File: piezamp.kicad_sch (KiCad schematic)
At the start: 54 parts, among them J3 Output (TRS), J4 Power_Conn, J5 Piezo A, J6 Piezo B, SW1 Power, SW2 Mode / Polarity, U1 NE5532DR, U2 NE5532DR

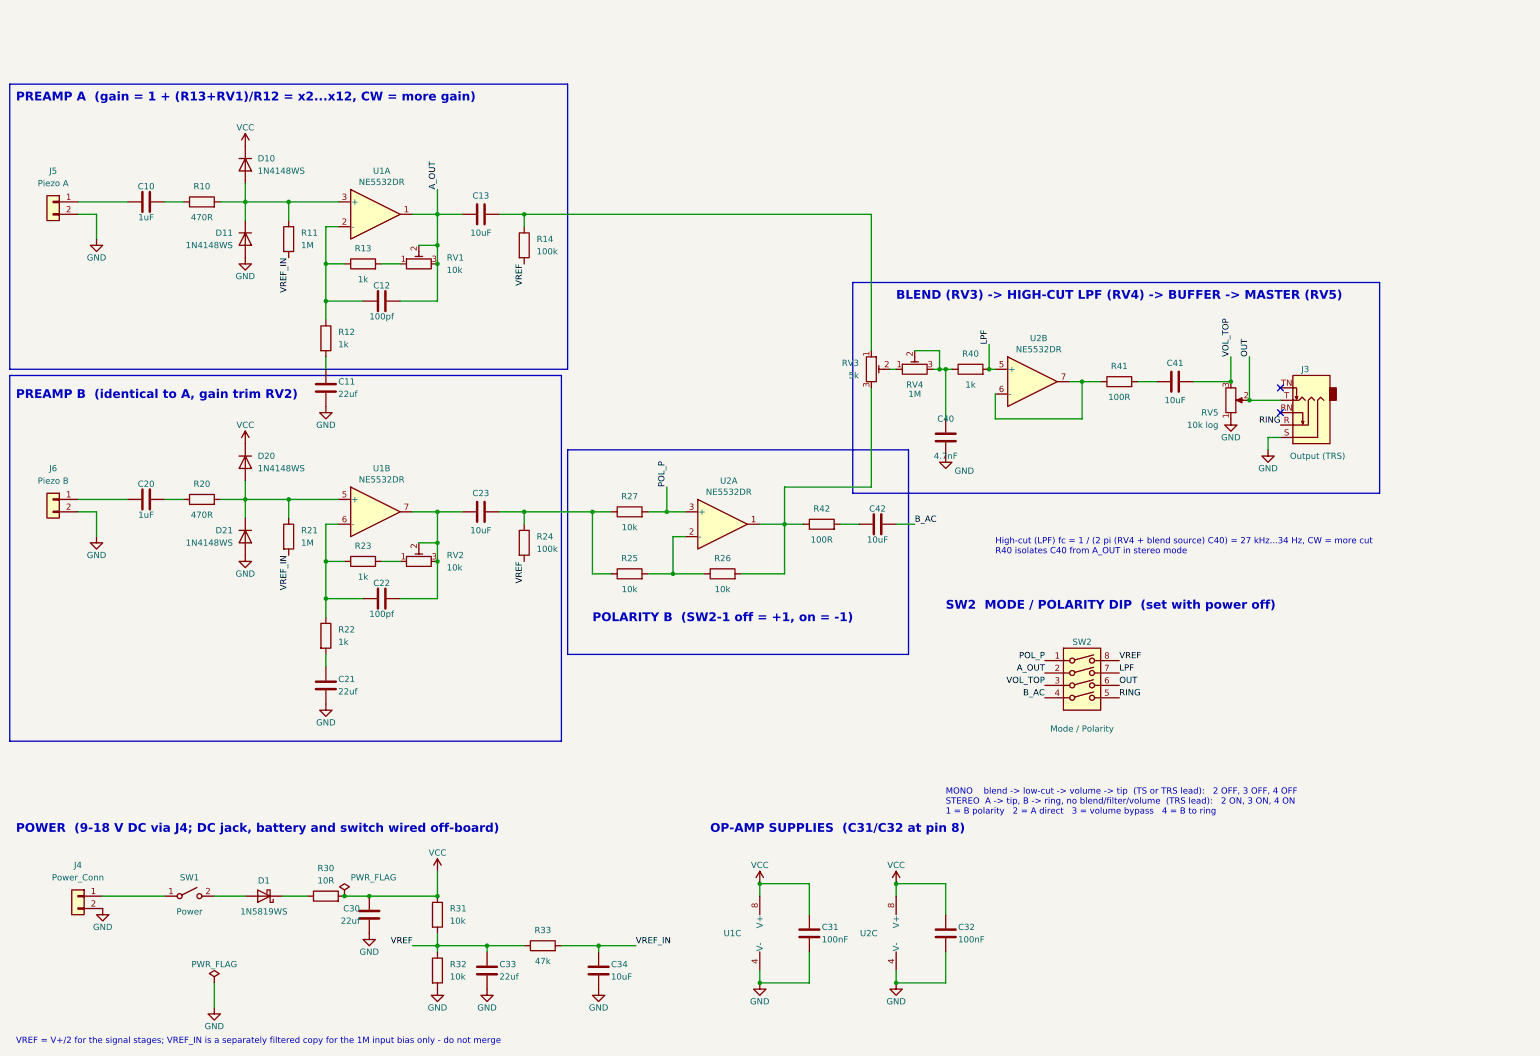
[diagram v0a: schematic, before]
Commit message: did some renders, annotated schematic
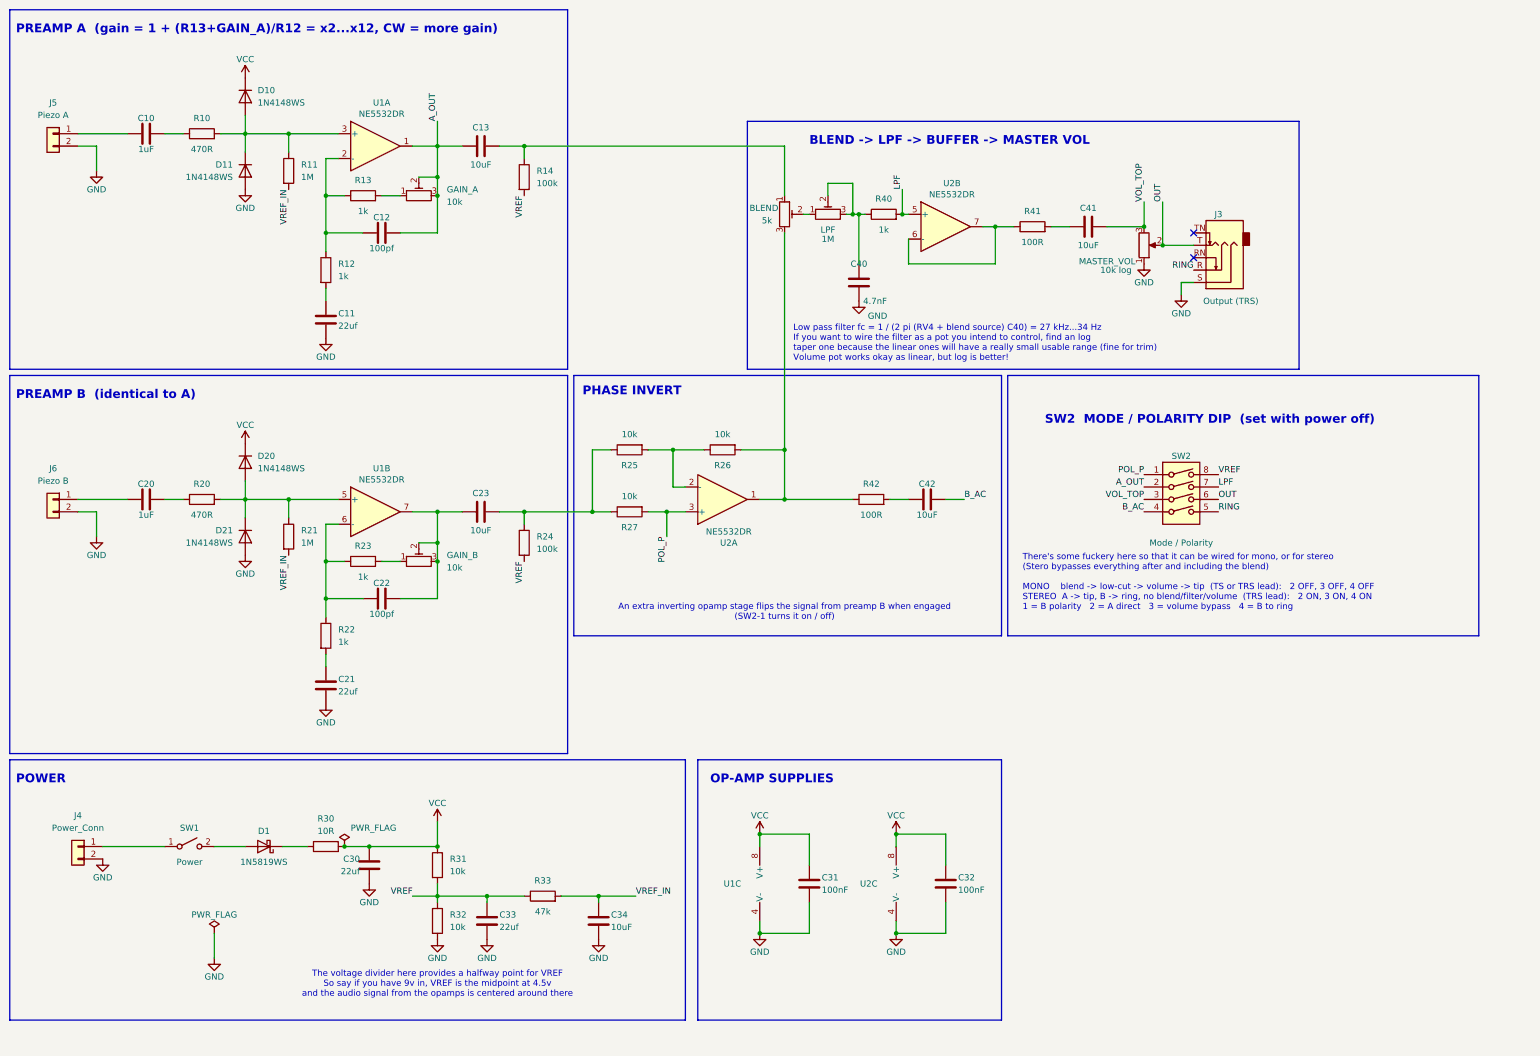
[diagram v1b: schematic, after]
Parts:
- renumbered RV3 to BLEND, RV1 to GAIN_A, RV2 to GAIN_B, RV4 to LPF, RV5 to MASTER_VOL
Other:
- note added: "An extra inverting opamp stage flips the signal from preamp B when engaged (SW2-1 turns it on / off)"
- note added: "BLEND -> LPF -> BUFFER -> MASTER VOL"
- note added: "Low pass filter fc = 1 / (2 pi (RV4 + blend source) C40) = 27 kHz...34 Hz If you want to wire the filter as a pot you intend to control, find an log taper one because the linear ones will have a really small usable range (fine for trim) Volume pot works okay as linear, but log is better!"
- note added: "OP-AMP SUPPLIES"
- note added: "PHASE INVERT"
- note added: "POWER"
- note added: "PREAMP A (gain = 1 + (R13+GAIN_A)/R12 = x2...x12, CW = more gain)"
- note added: "PREAMP B (identical to A)"
- note added: "The voltage divider here provides a halfway point for VREF So say if you have 9v in, VREF is the midpoint at 4.5v and the audio signal from the opamps is centered around there"
- note added: "There's some fuckery here so that it can be wired for mono, or for stereo (Stero bypasses everything after and including the blend) MONO blend -> low-cut -> volume -> tip (TS or TRS lead): 2 OFF, 3 OFF, 4 OFF STEREO A -> tip, B -> ring, no blend/filter/volume (TRS lead): 2 ON, 3 ON, 4 ON 1 = B polarity 2 = A direct 3 = volume bypass 4 = B to ring"
- note removed: "BLEND (RV3) -> HIGH-CUT LPF (RV4) -> BUFFER -> MASTER (RV5)"
- note removed: "High-cut (LPF) fc = 1 / (2 pi (RV4 + blend source) C40) = 27 kHz...34 Hz, CW = more cut R40 isolates C40 from A_OUT in stereo mode"
- note removed: "MONO blend -> low-cut -> volume -> tip (TS or TRS lead): 2 OFF, 3 OFF, 4 OFF STEREO A -> tip, B -> ring, no blend/filter/volume (TRS lead): 2 ON, 3 ON, 4 ON 1 = B polarity 2 = A direct 3 = volume bypass 4 = B to ring"
- note removed: "OP-AMP SUPPLIES (C31/C32 at pin 8)"
- note removed: "POLARITY B (SW2-1 off = +1, on = -1)"
- note removed: "POWER (9-18 V DC via J4; DC jack, battery and switch wired off-board)"
- note removed: "PREAMP A (gain = 1 + (R13+RV1)/R12 = x2...x12, CW = more gain)"
- note removed: "PREAMP B (identical to A, gain trim RV2)"
- note removed: "VREF = V+/2 for the signal stages; VREF_IN is a separately filtered copy for the 1M input bias only - do not merge"
- moved on the sheet: BLEND, C10, C11, C12, C13, C30, C31, C32, C33, C34, C40, C41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
